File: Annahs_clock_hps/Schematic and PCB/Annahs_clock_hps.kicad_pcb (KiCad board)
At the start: 2 copper layers, 140 x 90 mm, 70 parts, among them J1 Conn_01x06, J2 Power_inlet_vertical, J3 Conn_02x03_Odd_Even, Q1 NPN_2N3904_SOT23, SW1 Omron_B3F_SPST, SW2 Omron_B3F_SPST, SW3 Omron_B3F_SPST, SW4 Omron_B3F_SPST, SW5 Omron_B3F_SPST, SW6 Omron_B3F_SPST, U1 DS1307_DIP-8, U2 MAX7219, U3 L7805, U4 SC56-11EWA, U5 SC56-11EWA, Y1 Crystal_16MHz, Y2 Crystal_32768Hz

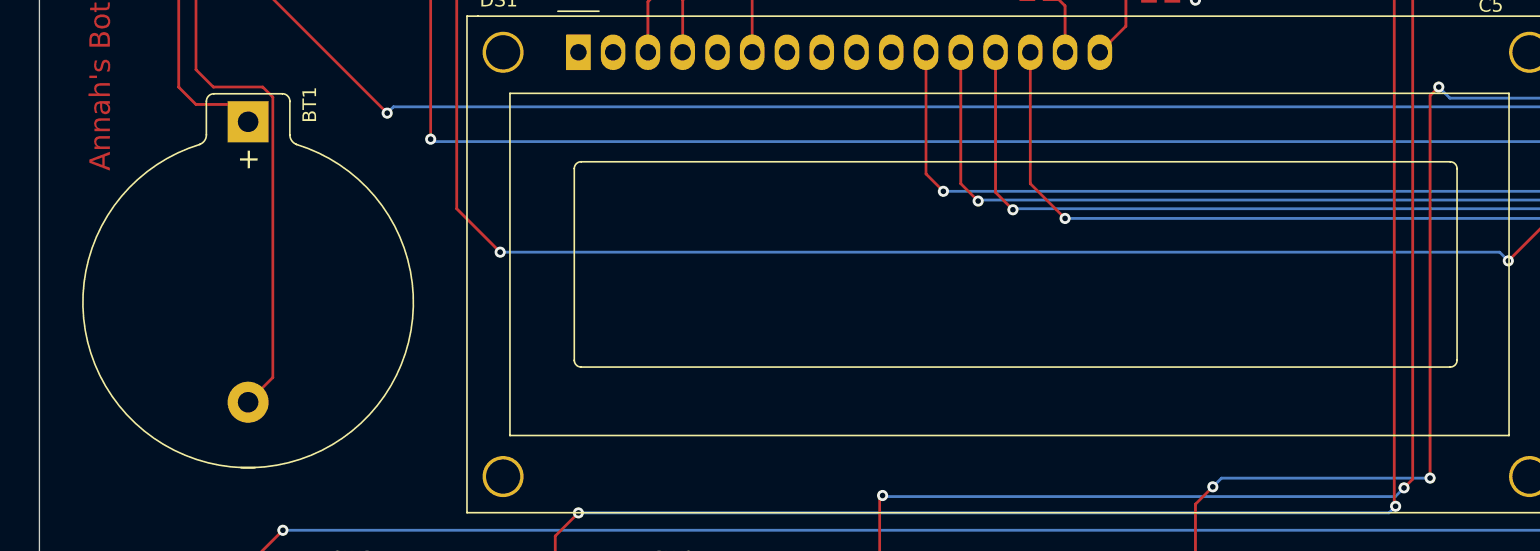
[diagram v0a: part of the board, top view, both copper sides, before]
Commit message: Updated Schematic and PCB
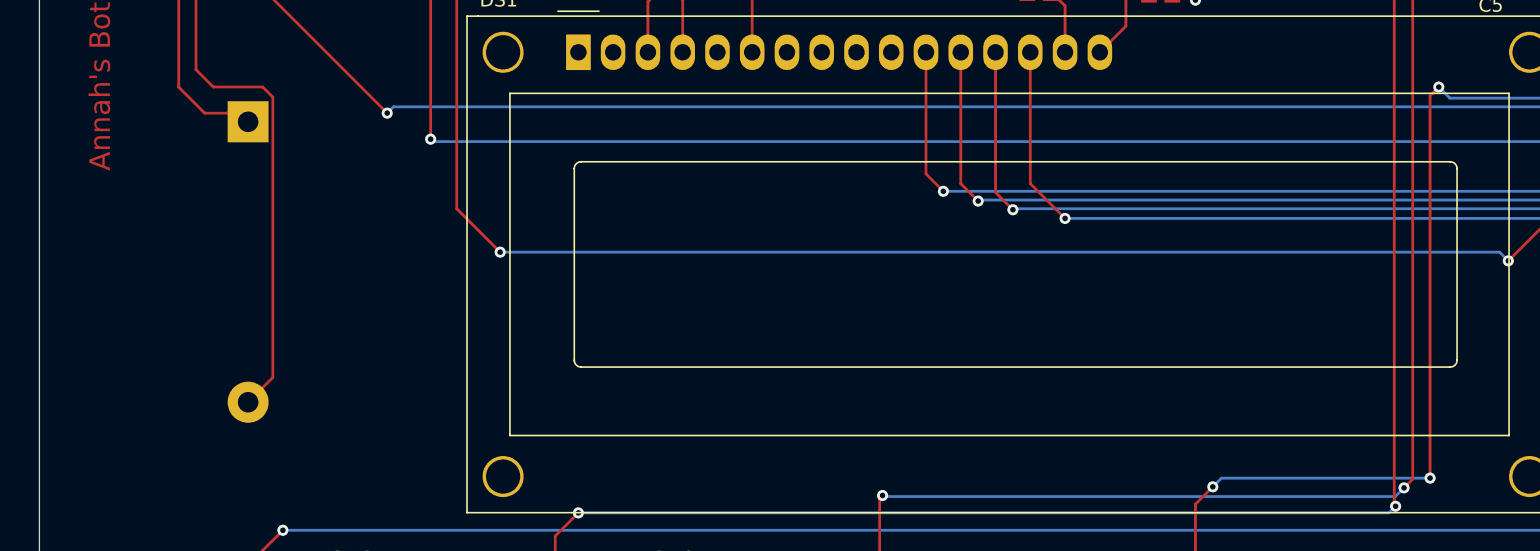
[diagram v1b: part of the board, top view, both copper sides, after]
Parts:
- BT1: moved to B.Cu
